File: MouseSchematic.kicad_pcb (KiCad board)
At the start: 2 copper layers, 125.4 x 125.4 mm, 67 parts, among them IC1 AZ1117IH-3.3TRG1, J1 Right Header, J2 Left Header, J4 JST1, J5 JST2, J6 Programming Header, Q1 IR Receiver, Q2 IR Receiver, Q3 IR Receiver, Q4 IR Receiver, Q5 MOSFET, Q6 MOSFET, Q7 MOSFET, Q8 MOSFET, SW1 Button, U1 STM32F205RGTx, U2 L293DD

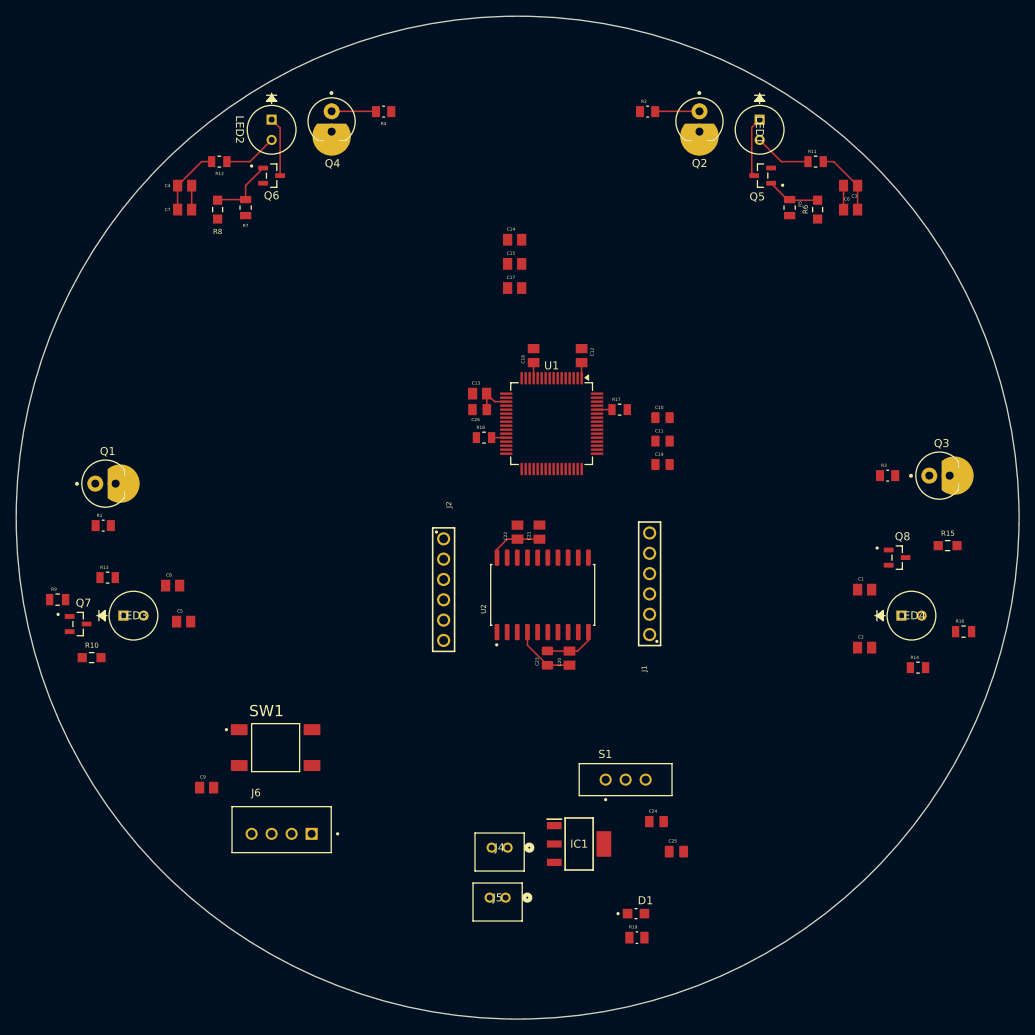
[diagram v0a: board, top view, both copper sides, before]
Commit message: Finished main layout of components still need to finish final touches and traces
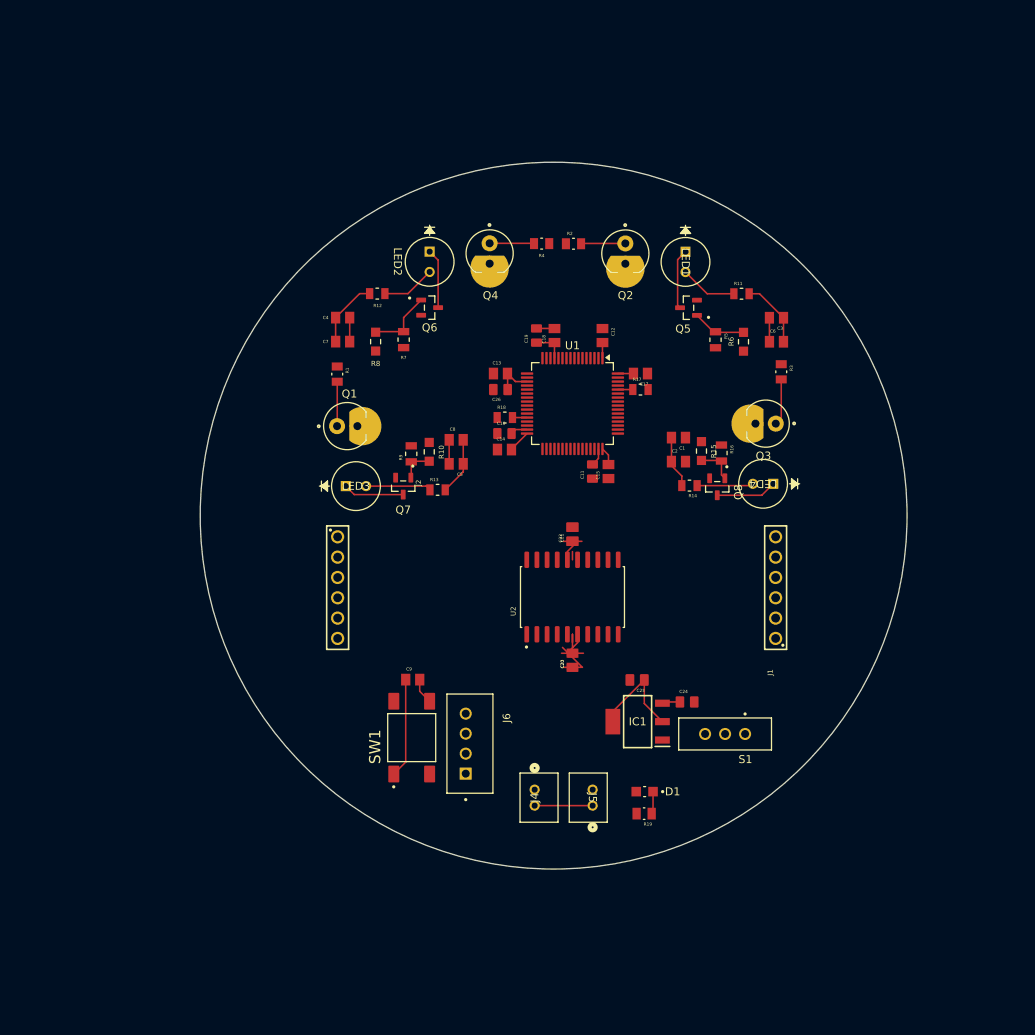
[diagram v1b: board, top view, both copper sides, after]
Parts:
- moved R10 49.4 mm to (141.2, 95.5), turned to -90 degrees
- moved R9 47.8 mm to (138.9, 95.8), turned to 90 degrees
- moved Q7 44.1 mm to (137.9, 99.8), turned to -90 degrees
- moved R13 42.7 mm to (142.2, 100.3)
- moved C8 39.9 mm to (144.6, 94.0)
- moved C5 39.4 mm to (144.6, 97.0), turned to 180 degrees
- moved R16 37.6 mm to (177.7, 95.7), turned to -90 degrees
- moved R14 36.5 mm to (173.7, 99.8), turned to 180 degrees
- moved R1 34.8 mm to (129.7, 85.8), turned to -90 degrees
- moved R15 33.0 mm to (175.2, 95.4), turned to -90 degrees
- moved C2 32.9 mm to (172.4, 96.8)
- moved LED3 32.2 mm to (130.8, 99.8)
- moved Q1 31.1 mm to (130.9, 92.3)
- moved C1 30.0 mm to (172.4, 93.8), turned to 180 degrees
- moved C9 29.1 mm to (139.1, 124.0)
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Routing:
- net 3V3: track 25.8 -> 61.8 mm
- net NRST: track 0.00 -> 12.4 mm
- net GND: track 13.9 -> 22.4 mm
- net Net-(LED3-Pad2): track 0.00 -> 8.17 mm
- net Net-(LED3-Pad1): track 0.00 -> 7.62 mm
- net Net-(LED4-Pad1): track 0.00 -> 7.59 mm
- net Net-(J4-Pad2): track 0.00 -> 7.25 mm
- net Net-(LED4-Pad2): track 0.00 -> 7.07 mm
- net PC4: track 0.00 -> 5.81 mm
- net PC5: track 0.00 -> 5.56 mm
- net Net-(Q8-Pad1): track 0.00 -> 4.87 mm
- net Net-(Q7-Pad1): track 0.00 -> 4.28 mm
- net Net-(D1-Pad1): track 0.00 -> 2.82 mm
- net Net-(IC1-INPUT): track 0.00 -> 2.25 mm
- net Net-(U1-VCAP_2): track 0.00 -> 2.25 mm
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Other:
- board size 125.4 x 125.4 mm -> 88.4 x 88.4 mm
